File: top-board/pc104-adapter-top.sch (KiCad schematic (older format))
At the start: 12 parts, among them J1 Conn_01x13_Male, J10 SAMTEC-SSW-126-01-G-D, J2 Conn_01x13_Male, J3 Conn_01x13_Male, J4 Conn_01x13_Male, J5 Conn_01x13_Male, J6 Conn_01x13_Male, J7 Conn_01x13_Male, J8 Conn_01x13_Male, J9 SAMTEC-SSW-126-01-G-D

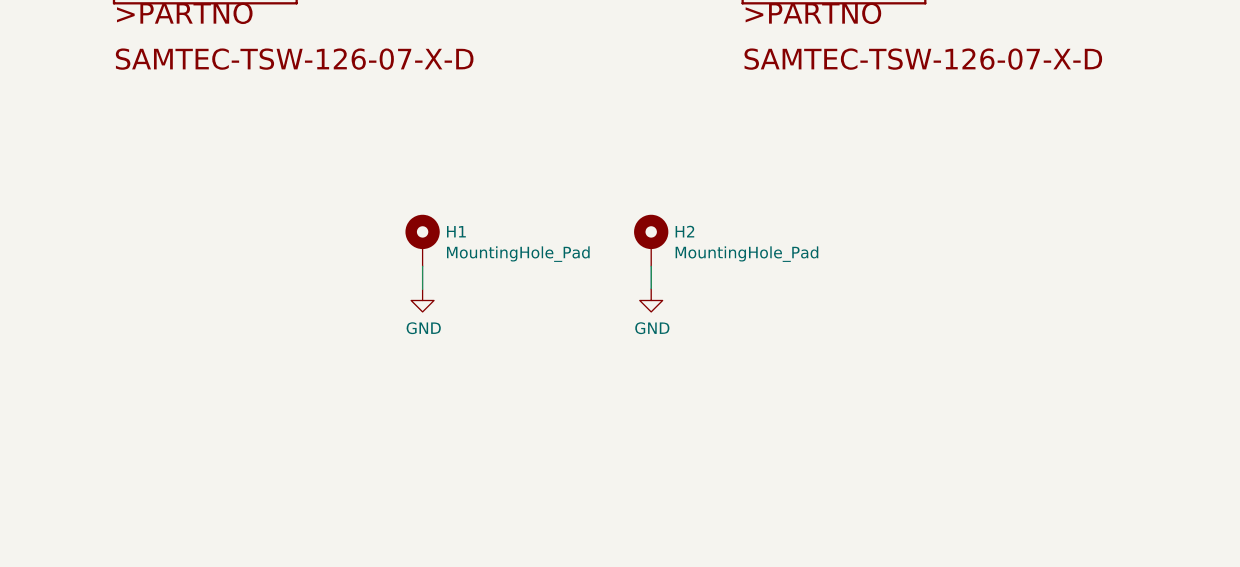
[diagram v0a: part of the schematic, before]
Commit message: top-board: Version 2.0 #13
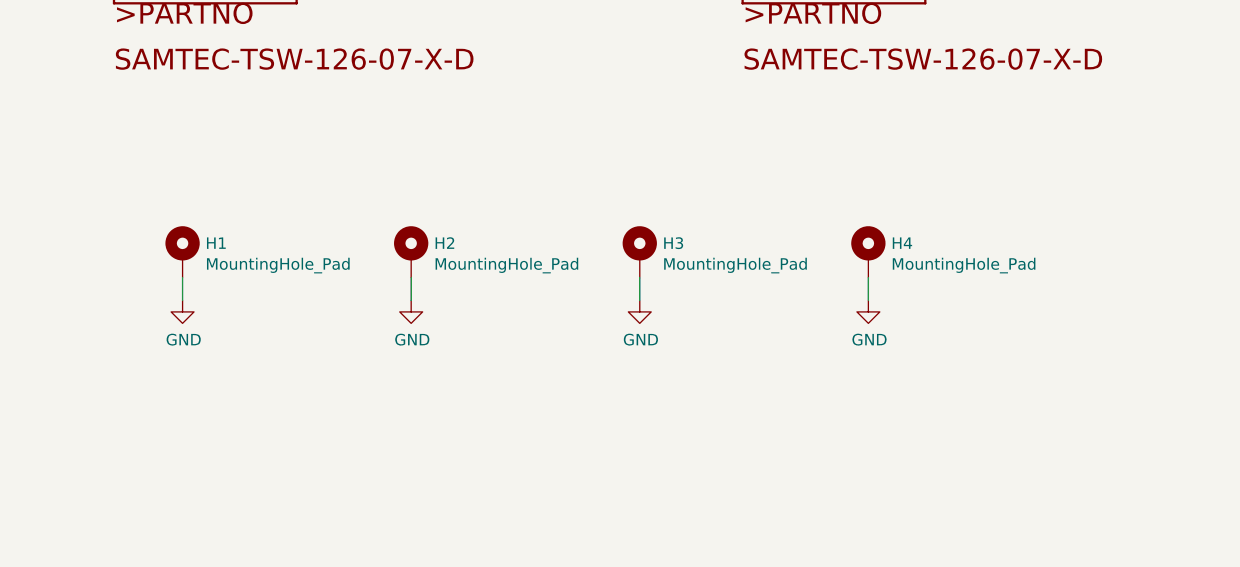
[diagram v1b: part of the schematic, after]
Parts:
- added H3, H4: MountingHole_Pad, MountingHole:MountingHole_3.2mm_M3_ISO14580_Pad, symbol Mechanical:MountingHole_Pad
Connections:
- net GND: now also H3.1, H4.1
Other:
- moved on the sheet: H1, H2
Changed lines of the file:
@@
 L Mechanical:MountingHole_Pad H1
 U 1 1 5F59E490
-P 7450 5250
-F 0 "H1" H 7550 5299 50  0000 L CNN
-F 1 "MountingHole_Pad" H 7550 5208 50  0000 L CNN
-F 2 "MountingHole:MountingHole_3.2mm_M3_ISO14580_Pad" H 7450 5250 50  0001 C CNN
-F 3 "~" H 7450 5250 50  0001 C CNN
-	1    7450 5250
+P 6400 5300
+F 0 "H1" H 6500 5349 50  0000 L CNN
+F 1 "MountingHole_Pad" H 6500 5258 50  0000 L CNN
+F 2 "MountingHole:MountingHole_3.2mm_M3_ISO14580_Pad" H 6400 5300 50  0001 C CNN
+F 3 "~" H 6400 5300 50  0001 C CNN
+	1    6400 5300
 	1    0    0    -1
 $EndComp
@@
 L Mechanical:MountingHole_Pad H2
 U 1 1 5F5A173F
-P 8450 5250
-F 0 "H2" H 8550 5299 50  0000 L CNN
-F 1 "MountingHole_Pad" H 8550 5208 50  0000 L CNN
-F 2 "MountingHole:MountingHole_3.2mm_M3_ISO14580_Pad" H 8450 5250 50  0001 C CNN
-F 3 "~" H 8450 5250 50  0001 C CNN
-	1    8450 5250
+P 7400 5300
+F 0 "H2" H 7500 5349 50  0000 L CNN
+F 1 "MountingHole_Pad" H 7500 5258 50  0000 L CNN
+F 2 "MountingHole:MountingHole_3.2mm_M3_ISO14580_Pad" H 7400 5300 50  0001 C CNN
+F 3 "~" H 7400 5300 50  0001 C CNN
+	1    7400 5300
 	1    0    0    -1
 $EndComp
@@
 L power:GND #PWR01
 U 1 1 5F5D55CB
-P 7450 5450
-F 0 "#PWR01" H 7450 5200 50  0001 C CNN
-F 1 "GND" H 7455 5277 50  0000 C CNN
-F 2 "" H 7450 5450 50  0001 C CNN
-F 3 "" H 7450 5450 50  0001 C CNN
-	1    7450 5450
+P 6400 5500
+F 0 "#PWR01" H 6400 5250 50  0001 C CNN
+F 1 "GND" H 6405 5327 50  0000 C CNN
+F 2 "" H 6400 5500 50  0001 C CNN
+F 3 "" H 6400 5500 50  0001 C CNN
+	1    6400 5500
 	1    0    0    -1
 $EndComp
@@
 L power:GND #PWR02
 U 1 1 5F5D6345
-P 8450 5450
-F 0 "#PWR02" H 8450 5200 50  0001 C CNN
-F 1 "GND" H 8455 5277 50  0000 C CNN
-F 2 "" H 8450 5450 50  0001 C CNN
-F 3 "" H 8450 5450 50  0001 C CNN
-	1    8450 5450
-	1    0    0    -1
-$EndComp
-Wire Wire Line
-	7450 5450 7450 5350
-Wire Wire Line
-	8450 5450 8450 5350
+P 7400 5500
+F 0 "#PWR02" H 7400 5250 50  0001 C CNN
+F 1 "GND" H 7405 5327 50  0000 C CNN
+F 2 "" H 7400 5500 50  0001 C CNN
+F 3 "" H 7400 5500 50  0001 C CNN
+	1    7400 5500
+	1    0    0    -1
+$EndComp
+Wire Wire Line
+	6400 5500 6400 5400
+Wire Wire Line
+	7400 5500 7400 5400
 Wire Wire Line
 	2200 2550 2000 2550
@@
 	1    0    0    -1
 $EndComp
+$Comp
+L Mechanical:MountingHole_Pad H3
+U 1 1 5F352380
+P 8400 5300
+F 0 "H3" H 8500 5349 50  0000 L CNN
+F 1 "MountingHole_Pad" H 8500 5258 50  0000 L CNN
+F 2 "MountingHole:MountingHole_3.2mm_M3_ISO14580_Pad" H 8400 5300 50  0001 C CNN
+F 3 "~" H 8400 5300 50  0001 C CNN
+	1    8400 5300
+	1    0    0    -1
+$EndComp
+$Comp
+L Mechanical:MountingHole_Pad H4
+U 1 1 5F352386
+P 9400 5300
+F 0 "H4" H 9500 5349 50  0000 L CNN
+F 1 "MountingHole_Pad" H 9500 5258 50  0000 L CNN
+F 2 "MountingHole:MountingHole_3.2mm_M3_ISO14580_Pad" H 9400 5300 50  0001 C CNN
+F 3 "~" H 9400 5300 50  0001 C CNN
+	1    9400 5300
+	1    0    0    -1
+$EndComp
+$Comp
+L power:GND #PWR0101
+U 1 1 5F35238C
+P 8400 5500
+F 0 "#PWR0101" H 8400 5250 50  0001 C CNN
+F 1 "GND" H 8405 5327 50  0000 C CNN
+F 2 "" H 8400 5500 50  0001 C CNN
+F 3 "" H 8400 5500 50  0001 C CNN
+	1    8400 5500
+	1    0    0    -1
+$EndComp
+$Comp
+L power:GND #PWR0102
+U 1 1 5F352392
+P 9400 5500
+F 0 "#PWR0102" H 9400 5250 50  0001 C CNN
+F 1 "GND" H 9405 5327 50  0000 C CNN
+F 2 "" H 9400 5500 50  0001 C CNN
+F 3 "" H 9400 5500 50  0001 C CNN
+	1    9400 5500
+	1    0    0    -1
+$EndComp
+Wire Wire Line
+	8400 5500 8400 5400
+Wire Wire Line
+	9400 5500 9400 5400
 $EndSCHEMATC
